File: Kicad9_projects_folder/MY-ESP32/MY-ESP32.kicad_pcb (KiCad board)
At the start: 4 copper layers, 97.3 x 90.9 mm, 108 parts, among them Q1 2N3904S-RTK/PS, Q2 2N3904S-RTK/PS, Q3 N-MOSFET-ENH-2N7002, Q4 P-MOSFET-ENH-BSS84LT1G, Q5 PMOSFET-DMP1045U-7, SW1 BOOT, SW2 RESET, U1 USBLC6-2SC6, U10 USB-C_Connector, U2 Screw_Terminal_KF301_1x02, U3 CP2102N-Axx-xQFN28, U5 TPS63001DRCR, U7 LTC4121EUD#TRPBF

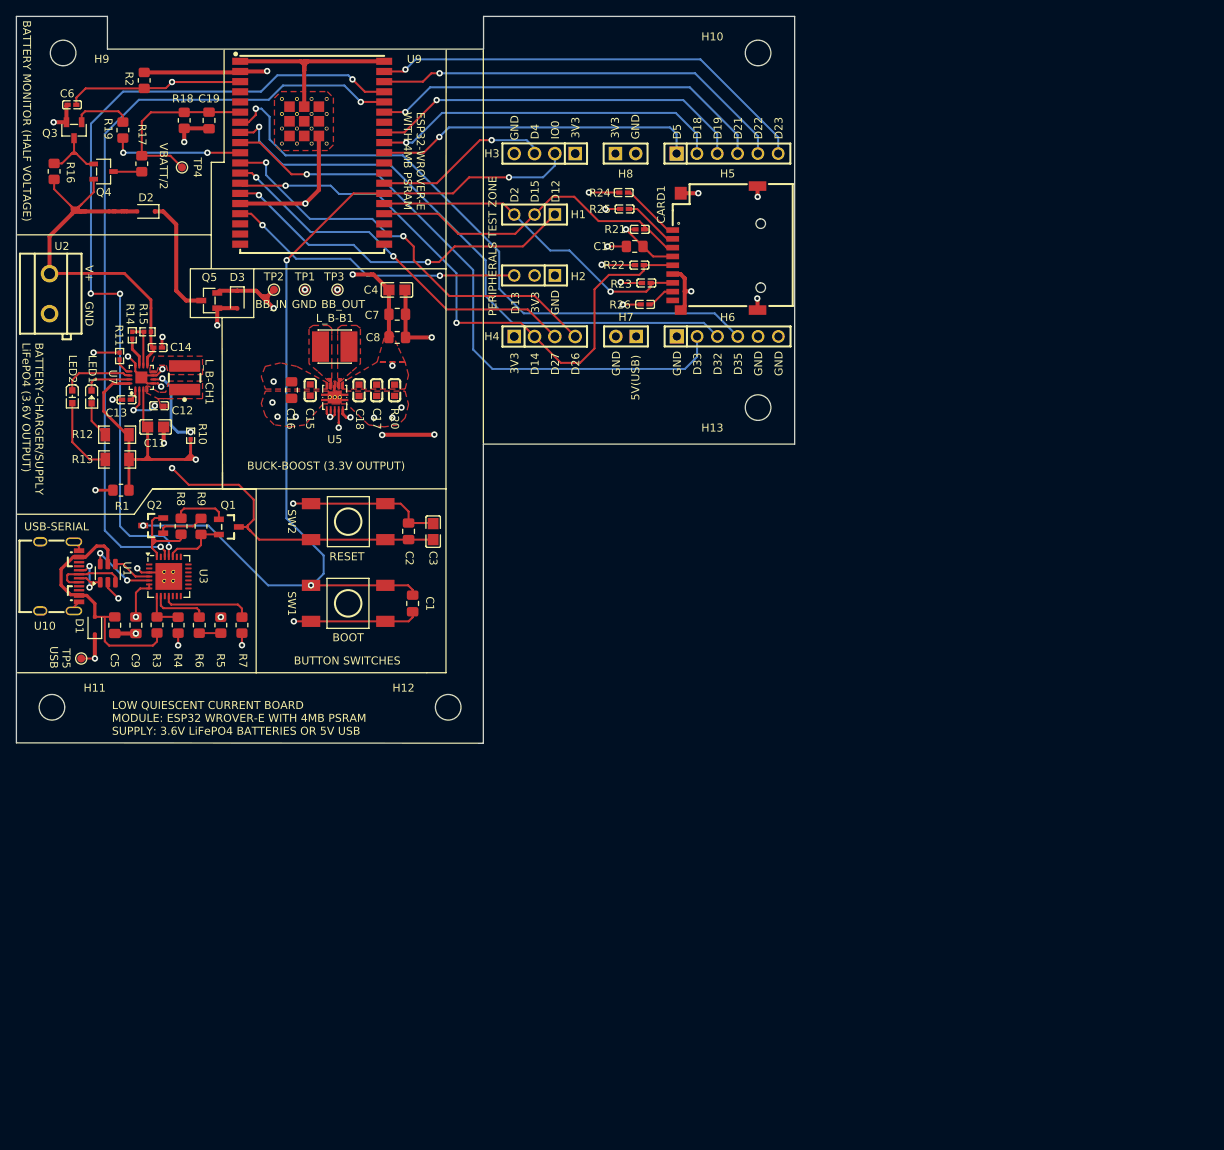
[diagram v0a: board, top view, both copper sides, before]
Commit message: Second commit
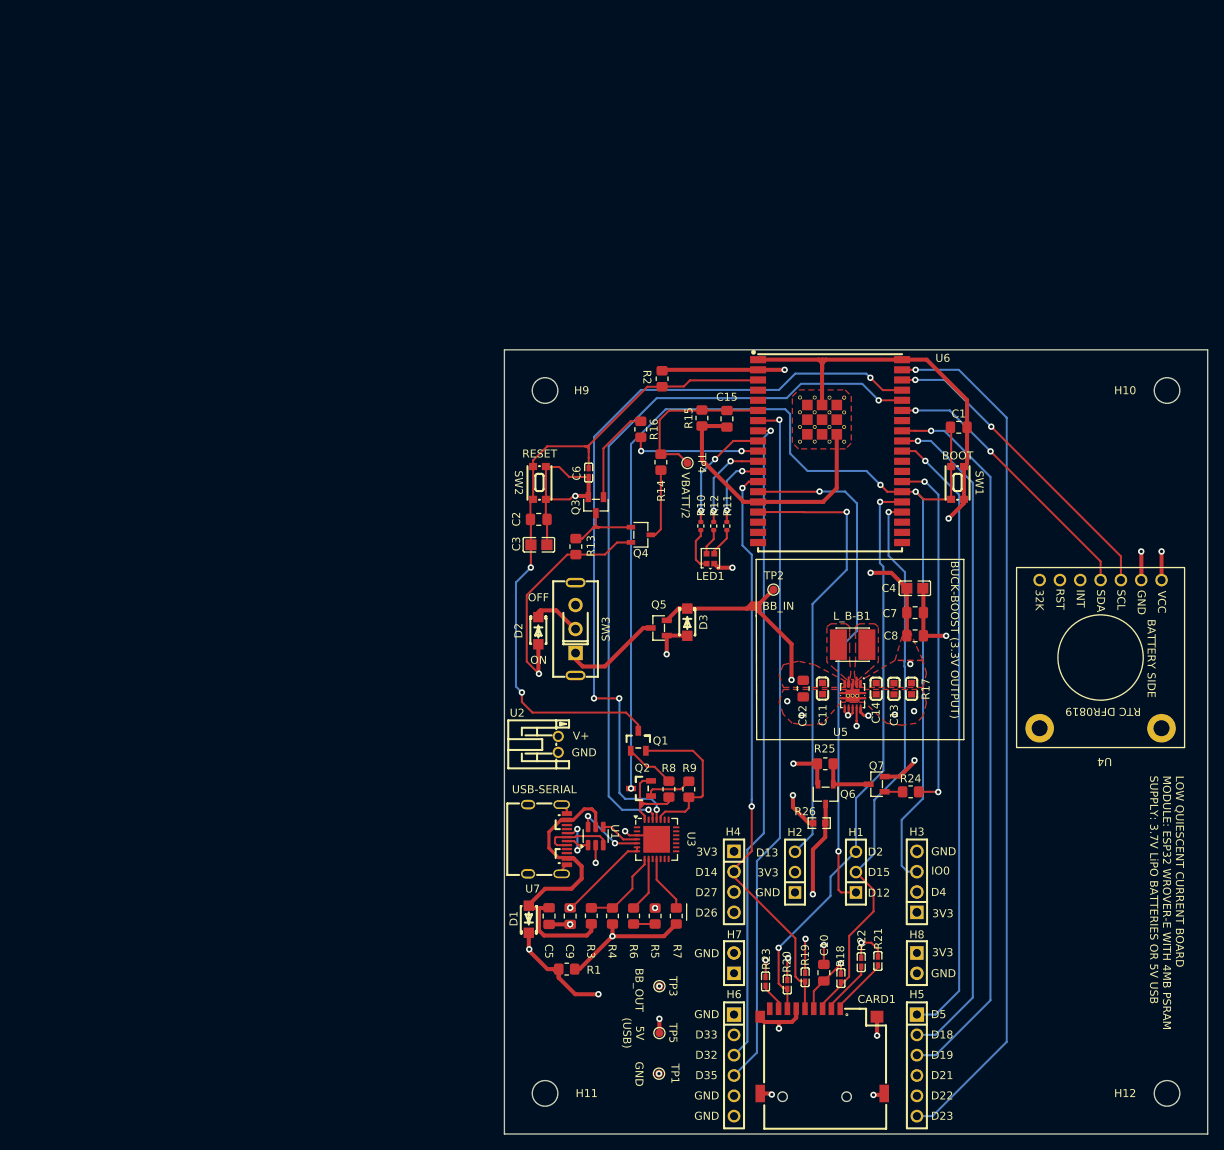
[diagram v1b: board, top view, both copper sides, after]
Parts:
- removed the ? at (44.2, 87.1)
- removed the ? at (59.7, 33.6)
- removed the ? at (63.4, 31.7)
- removed the ? at (43.1, 87.1)
- removed the ? at (57.8, 33.6)
- removed the ? at (63.4, 28.0)
- removed the ? at (64.4, 65.3)
- removed the ? at (61.5, 29.9)
- removed the ? at (57.8, 29.9)
- removed the ? at (61.5, 28.0)
- removed the ? at (61.5, 33.6)
- removed the ? at (57.8, 31.7)
- removed the ? at (57.8, 28.0)
- removed the ? at (65.0, 65.3)
- removed the ? at (63.4, 29.9)
- removed the ? at (59.7, 28.0)
- removed the ? at (59.7, 31.7)
- removed the ? at (44.2, 88.3)
- removed the ? at (63.8, 65.3)
- removed the ? at (59.7, 29.9)
- removed the ? at (61.5, 31.7)
- removed the ? at (43.1, 88.3)
- removed the ? at (63.4, 33.6)
- removed the C15 at (61.3, 64.4)
- removed C16: 104, Capacitor_SMD:C_0805_2012Metric_Pad1.18x1.45mm_HandSolder
- removed C17: 10uF ±10% 10V, My_Personal_Footprints_Library:CL10A106KP8NNNC
- removed C18: 4.7uF, My_Personal_Footprints_Library:CL10A475KP8NNNC
- removed H13: MountingHole, MountingHole:MountingHole_3.2mm_M3
- removed LED2: EMERALD, My_Personal_Footprints_Library:LED_EMERALD_20mA_FC-D1608UGK-520D10
- removed L_B-CH1: 47uH±20% - 680mA, My_Personal_Footprints_Library:ind_47uH_LPS4018-473MRC
- removed the U7 at (40.2, 62.8)
- added ?: , , F.Cu at (126.2, 70.9)
- added ?: , , F.Cu at (124.4, 65.3)
- added ?: , , F.Cu at (128.1, 70.9)
- added ?: , , F.Cu at (126.2, 69.0)
- added ?: , , F.Cu at (122.5, 65.3)
- added ?: , , F.Cu at (122.5, 67.2)
- added ?: , , F.Cu at (126.2, 67.2)
- added ?: , , F.Cu at (122.5, 70.9)
- added ?: , , F.Cu at (124.4, 67.2)
- added ?: , , F.Cu at (128.1, 69.0)
- added ?: , , F.Cu at (124.4, 70.9)
- added ?: , , F.Cu at (129.7, 102.6)
- added ?: , , F.Cu at (128.5, 102.6)
- added ?: , , F.Cu at (128.1, 65.4)
- added ?: , , F.Cu at (124.4, 69.0)
- added ?: , , F.Cu at (126.2, 65.4)
- added ?: , , F.Cu at (122.5, 69.0)
- added ?: , , F.Cu at (128.1, 67.2)
- added ?: , , F.Cu at (129.1, 102.6)
- added Q6: P-MOSFET-ENH-BSS84LT1G, My_Personal_Footprints_Library:BSS84LT1G, F.Cu at (125.7, 114.9)
- added Q7: N-MOSFET-ENH-2N7002, My_Personal_Footprints_Library:2N7002, F.Cu at (132.1, 113.7)
- added SW3: SPDT, My_Personal_Footprints_Library:SS-12F49-G050, F.Cu at (94.5, 94.3)
- added U4: DFR0819, My_Personal_Footprints_Library:DFR0819, F.Cu at (160.6, 97.8)
- C11: value 10uF ±10% 25V -> 10uF ±10% 10V; footprint My_Personal_Footprints_Library:CAP_10uF_CL21A106KAYNNNE -> My_Personal_Footprints_Library:CL10A106KP8NNNC
- C12: value 22nF -> 104; footprint My_Personal_Footprints_Library:CAP_22nF_0402B223K500NT -> Capacitor_SMD:C_0805_2012Metric_Pad1.18x1.45mm_HandSolder
- C13: value 2.2uF ±10% 25V -> 10uF ±10% 10V; footprint My_Personal_Footprints_Library:CAP_2.2uF_GRM155R61E225KE11D -> My_Personal_Footprints_Library:CL10A106KP8NNNC
- C14: value 22uF ±20% 6.3V -> 4.7uF; footprint My_Personal_Footprints_Library:CM05X5R226M06AH080 -> My_Personal_Footprints_Library:CL10A475KP8NNNC
- CARD1: value micro SD Card slot TF PUSH -> micro SD-CARD TF PUSH
- D1, D2, D3: value BAT760-7 -> RB168MM-40TR; footprint Diode_SMD:D_SOD-323F -> My_Personal_Footprints_Library:RB168MM-40TR
- LED1: value RED -> E6C0606RGBC3UDA; footprint My_Personal_Footprints_Library:LED0603-RD_RED -> My_Personal_Footprints_Library:E6C0606RGBC3UDA
- R10: value 10kΩ ±1% 62.5mW -> 150Ω ±1% 62.5mW; footprint My_Personal_Footprints_Library:RES_10K_0402WGF1002TCE -> Resistor_SMD:R_0402_1005Metric
- R11: value 3kΩ ±1% 62.5mW -> 36Ω ±1% 62.5mW; footprint My_Personal_Footprints_Library:FRC04002F3001TS -> Resistor_SMD:R_0402_1005Metric
- R12: value 604Ω -> 36Ω ±1% 62.5mW; footprint My_Personal_Footprints_Library:RTT066040FTP -> Resistor_SMD:R_0402_1005Metric
- R13: value 604Ω -> 10K; footprint My_Personal_Footprints_Library:RTT066040FTP -> Resistor_SMD:R_0805_2012Metric_Pad1.20x1.40mm_HandSolder
- R14: value 1.78MΩ ±1% 62.5mW -> 10K; footprint My_Personal_Footprints_Library:RC0402FR-071M78L -> Resistor_SMD:R_0805_2012Metric_Pad1.20x1.40mm_HandSolder
- R15: value 887kΩ -> 10K; footprint My_Personal_Footprints_Library:RC0402FR-07887KL -> Resistor_SMD:R_0805_2012Metric_Pad1.20x1.40mm_HandSolder
- R16: value 10K -> 100
- R17: value 10K -> 220Ω; footprint Resistor_SMD:R_0805_2012Metric_Pad1.20x1.40mm_HandSolder -> My_Personal_Footprints_Library:0603WAJ0221T5E
- R18: value 10K -> 7.5kΩ; footprint Resistor_SMD:R_0805_2012Metric_Pad1.20x1.40mm_HandSolder -> My_Personal_Footprints_Library:0603WAF7501T5E
- R19: value 100 -> 7.5kΩ; footprint Resistor_SMD:R_0805_2012Metric_Pad1.20x1.40mm_HandSolder -> My_Personal_Footprints_Library:0603WAF7501T5E
- R20: value 220Ω -> 7.5kΩ; footprint My_Personal_Footprints_Library:0603WAJ0221T5E -> My_Personal_Footprints_Library:0603WAF7501T5E
- R24: value 7.5kΩ -> 100; footprint My_Personal_Footprints_Library:0603WAF7501T5E -> Resistor_SMD:R_0805_2012Metric_Pad1.20x1.40mm_HandSolder
- R25: value 7.5kΩ -> 10K; footprint My_Personal_Footprints_Library:0603WAF7501T5E -> Resistor_SMD:R_0805_2012Metric_Pad1.20x1.40mm_HandSolder
- R26: value 7.5kΩ -> 4.7kΩ ±1% 100mW; footprint My_Personal_Footprints_Library:0603WAF7501T5E -> My_Personal_Footprints_Library:0603WAF4701T5E
- SW1: value BOOT -> ~; footprint My_Personal_Footprints_Library:SW_1TS005F-2500-5001 -> My_Personal_Footprints_Library:KMR211NGLFS
- SW2: value RESET -> ~; footprint My_Personal_Footprints_Library:SW_1TS005F-2500-5001 -> My_Personal_Footprints_Library:KMR211NGLFS
- U2: value Screw_Terminal_KF301_1x02 -> ~; footprint My_Personal_Footprints_Library:Screw_Terminal_KF301_1x02 -> My_Personal_Footprints_Library:CONN-TH_S2B-PH-K-S-GW
- moved R19 136.0 mm to (123.2, 137.8), turned to 90 degrees
- moved R18 135.0 mm to (127.7, 137.9)
- moved R17 116.5 mm to (136.5, 101.7), turned to 90 degrees
- moved H5 116.4 mm to (137.2, 148.8), turned to -90 degrees
- moved H8 107.5 mm to (137.2, 136.0), turned to -90 degrees
- moved TP1 107.5 mm to (104.9, 149.9), turned to 0 degrees
- moved C13 102.5 mm to (134.3, 101.8), turned to 90 degrees
- moved H3 102.2 mm to (137.2, 125.9), turned to 90 degrees
- moved H12 102.0 mm to (168.4, 152.3)
- moved CARD1 101.3 mm to (125.3, 147.0), turned to 0 degrees
- moved C14 99.4 mm to (132.1, 101.7), turned to 90 degrees
- moved R21 96.2 mm to (132.3, 135.8), turned to 90 degrees
- moved TP3 95.9 mm to (105.0, 138.9), turned to -90 degrees
- moved C10 93.8 mm to (125.5, 137.2), turned to -90 degrees
- moved H1 91.5 mm to (129.5, 124.7), turned to 90 degrees
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- renumbered C19 to C15, U9 to U6, U10 to U7
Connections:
- C10 pad 2: +3V3 -> /micro_SD-CARD_enable/3V3_Input_to_micro_SD-CARD
- C11 pad 2: EXT_5V -> /Buck-Boost3.3V/Buck-Boost_INPUT
- C12 pad 1: Net-(U7-SW) -> /Buck-Boost3.3V/Buck-Boost_INPUT
- C12 pad 2: Net-(U7-BOOST) -> GND
- C13 pad 1: Net-(U7-INTVcc) -> GND
- C13 pad 2: GND -> +3V3
- C14 pad 2: /Battery_Charger_LiFePO4_3.6V/Battery_Charger_OUTPUT -> +3V3
- CARD1 pad 4: +3V3 -> /micro_SD-CARD_enable/3V3_Input_to_micro_SD-CARD
- D2 pad 1: VBAT -> Net-(D2-C)
- D2 pad 2: /Battery_Charger_LiFePO4_3.6V/Battery_Charger_OUTPUT -> /Battery_Voltage_Monitor_with_MOSFETS/V_Batt_Monitor_INPUT
- H3 pad 2: IO0 -> GND
- H3 pad 3: D4 -> IO0
- H4 pad 3: D27 -> +3V3
- H4 pad 4: D26 -> GND
- H5 pad 4: D21 -> +3V3
- H5 pad 5: D22 -> GND
- H6 pad 2: D33 -> EXT_5V
- LED1 pad 1: Net-(LED1-K) -> Net-(LED1-B)
- LED1 pad 2: Net-(LED1-A) -> +3V3
- Q4 pad 2: /Battery_Charger_LiFePO4_3.6V/Battery_Charger_OUTPUT -> /Battery_Voltage_Monitor_with_MOSFETS/V_Batt_Monitor_INPUT
- R10 pad 1: Net-(U7-MPPT) -> Net-(LED1-R)
- R10 pad 2: EXT_5V -> D33
- R11 pad 1: GND -> D27
- R11 pad 2: Net-(U7-PROG) -> Net-(LED1-B)
- R12 pad 1: Net-(LED1-A) -> D26
- R12 pad 2: EXT_5V -> Net-(LED1-G)
- R13 pad 1: Net-(LED2-A) -> Net-(Q3-D)
- R13 pad 2: EXT_5V -> /Battery_Voltage_Monitor_with_MOSFETS/V_Batt_Monitor_INPUT
- R14 pad 1: Net-(U7-FB) -> D34
- R14 pad 2: Net-(U7-FBG) -> Net-(Q4-D)
- R15 pad 1: /Battery_Charger_LiFePO4_3.6V/Battery_Charger_OUTPUT -> GND
- R15 pad 2: Net-(U7-FB) -> D34
- R16 pad 1: Net-(Q3-D) -> Net-(Q3-G)
- R16 pad 2: /Battery_Charger_LiFePO4_3.6V/Battery_Charger_OUTPUT -> D25
- R17 pad 1: D34 -> GND
- R17 pad 2: Net-(Q4-D) -> +3V3
- R18 pad 1: GND -> D15
- R18 pad 2: D34 -> /micro_SD-CARD_enable/3V3_Input_to_micro_SD-CARD
- R19 pad 1: Net-(Q3-G) -> D14
- R19 pad 2: D25 -> /micro_SD-CARD_enable/3V3_Input_to_micro_SD-CARD
- R20 pad 1: GND -> D2
- R20 pad 2: +3V3 -> /micro_SD-CARD_enable/3V3_Input_to_micro_SD-CARD
- R21 pad 1: D15 -> Net-(CARD1-DAT2)
- R21 pad 2: +3V3 -> /micro_SD-CARD_enable/3V3_Input_to_micro_SD-CARD
- R22 pad 1: D14 -> Net-(CARD1-CD/DAT3)
- R22 pad 2: +3V3 -> /micro_SD-CARD_enable/3V3_Input_to_micro_SD-CARD
- R23 pad 1: D2 -> Net-(CARD1-DAT1)
- R23 pad 2: +3V3 -> /micro_SD-CARD_enable/3V3_Input_to_micro_SD-CARD
- R24 pad 1: Net-(CARD1-DAT2) -> Net-(Q7-G)
- R24 pad 2: +3V3 -> D4
- R25 pad 1: Net-(CARD1-CD/DAT3) -> Net-(Q6-G)
- R26 pad 1: Net-(CARD1-DAT1) -> GND
- R26 pad 2: +3V3 -> /micro_SD-CARD_enable/3V3_Input_to_micro_SD-CARD
- SW1 pad 2: IO0 -> GND
- SW1 pad 3: GND -> IO0
- SW2 pad 2: ENA -> GND
- SW2 pad 3: GND -> ENA
- U2 pad 1: /Battery_Charger_LiFePO4_3.6V/Battery_Charger_OUTPUT -> /Battery_Voltage_Monitor_with_MOSFETS/V_Batt_Monitor_INPUT
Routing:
- net /micro_SD-CARD_enable/3V3_Input_to_micro_SD-CARD: track 0.00 -> 66.9 mm, vias 0 -> 6
- net D33: track 77.8 -> 14.9 mm, vias 1 -> 2
- net /Battery_Charger_LiFePO4_3.6V/Battery_Charger_OUTPUT: track 59.7 -> 0.00 mm
- net EXT_5V: track 164.0 -> 106.1 mm, vias 5 -> 4
- net D23: track 56.0 -> 108.7 mm
- net D19: track 47.5 -> 91.0 mm
- net D26: track 52.8 -> 11.9 mm
- net D18: track 44.2 -> 84.6 mm
- net /Battery_Voltage_Monitor_with_MOSFETS/V_Batt_Monitor_INPUT: track 0.00 -> 38.8 mm, vias 0 -> 1
- net D27: track 47.8 -> 9.57 mm
- net D5: track 40.6 -> 78.0 mm
- net GND: track 150.3 -> 182.0 mm, vias 32 -> 21
- net D2: track 41.8 -> 73.2 mm, vias 1 -> 2
- net IO0: track 120.9 -> 152.0 mm, vias 4 -> 3
- net D15: track 42.5 -> 71.6 mm, vias 0 -> 1
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- removed copper zone on F.Cu, net Net-(U7-CHGSNS)
- removed copper zone on F.Cu, net Net-(U7-SW)
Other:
- board size 97.3 x 90.9 mm -> 87.9 x 98 mm
- board text added: "5V (USB)"
- board text added: "LOW QUIESCENT CURRENT BOARD MODULE: ESP32 WROVER-E WITH 4MB PSRAM SUPPLY: 3.7V LiPO BATTERIES OR 5V USB"
- board text added: "OFF"
- board text added: "ON"
- board text removed: "5V(USB)"
- board text removed: "BATTERY MONITOR (HALF VOLTAGE)"
- board text removed: "BATTERY-CHARGER/SUPPLY LiFePO4 (3.6V OUTPUT)"
- board text removed: "BUTTON SWITCHES"
- board text removed: "ESP32-WROVER-E WITH 4MB PSRAM"
- board text removed: "LOW QUIESCENT CURRENT BOARD MODULE: ESP32 WROVER-E WITH 4MB PSRAM SUPPLY: 3.6V LiFePO4 BATTERIES OR 5V USB"
- board text removed: "PERIPHERALS TEST ZONE"
- board text removed: "USB"
